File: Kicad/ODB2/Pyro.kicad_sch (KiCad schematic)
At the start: 35 parts

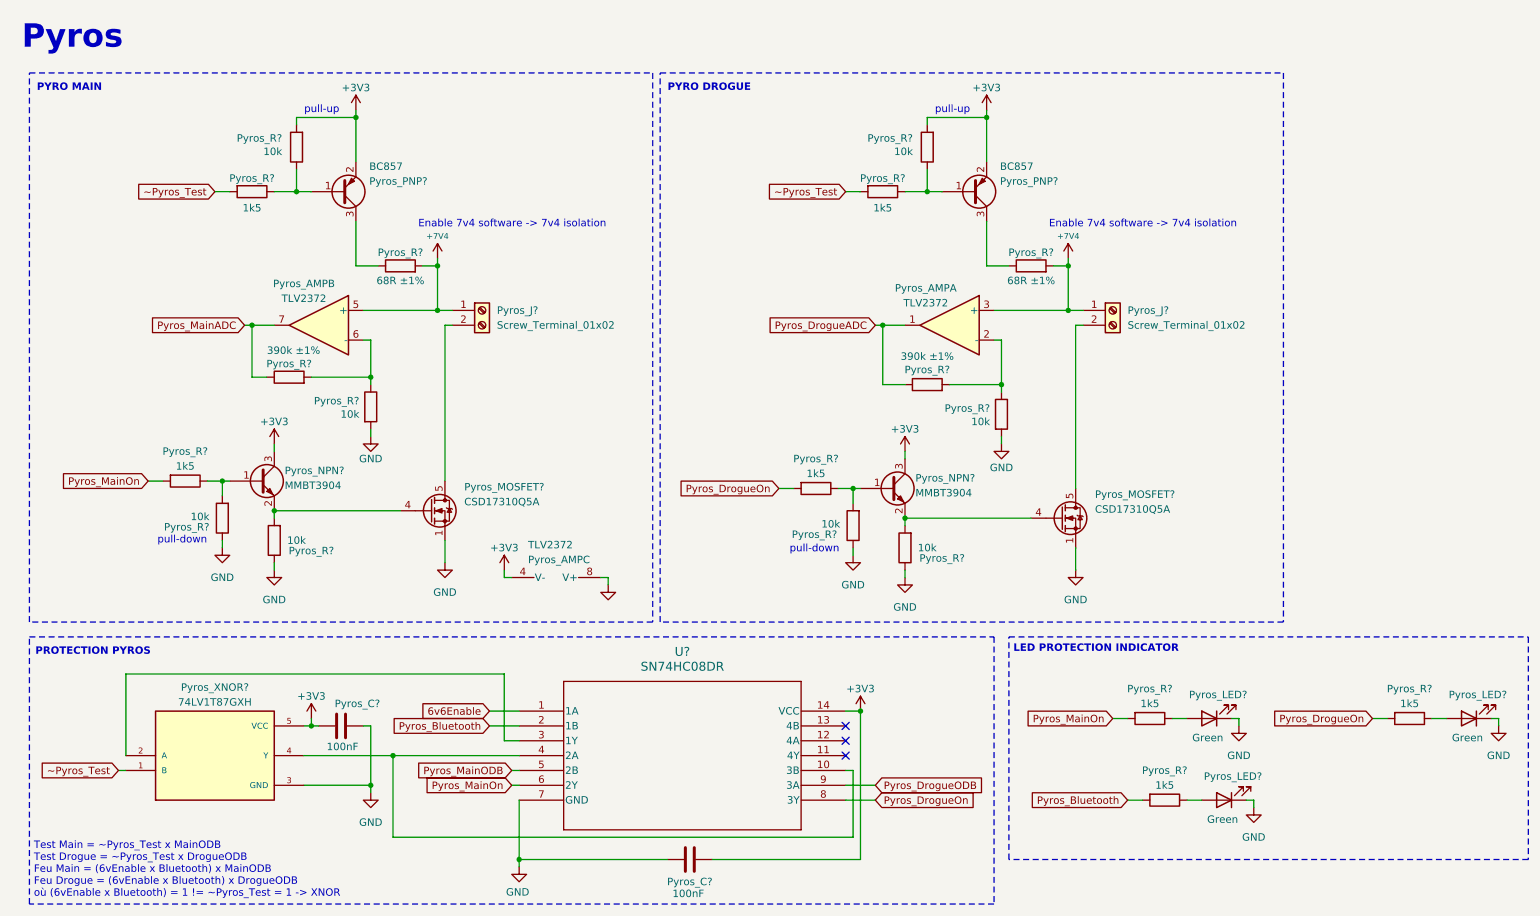
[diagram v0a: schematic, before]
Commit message: fix amp
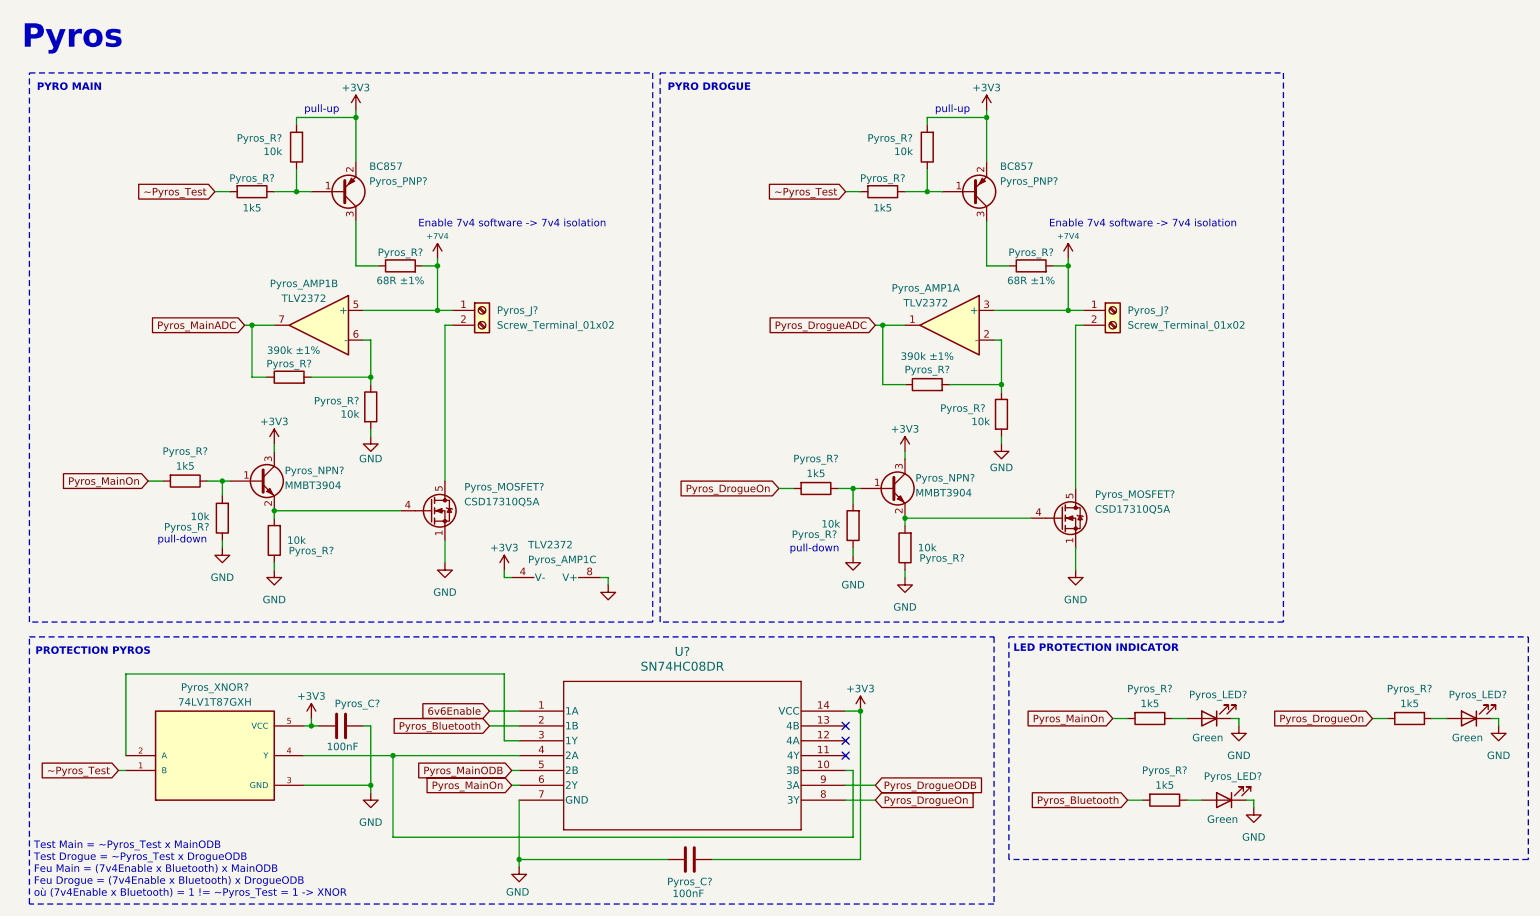
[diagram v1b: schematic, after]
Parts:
- Pyros_AMP1: renamed from Pyros_AMP; footprint (none) -> Package_SO:SOIC-8-1EP_3.9x4.9mm_P1.27mm_EP2.41x3.81mm
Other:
- note added: "Test Main = ~Pyros_Test x MainODB Test Drogue = ~Pyros_Test x DrogueODB Feu Main = (7v4Enable x Bluetooth) x MainODB Feu Drogue = (7v4Enable x Bluetooth) x DrogueODB où (7v4Enable x Bluetooth) = 1 != ~Pyros_Test = 1 -> XNOR"
- note removed: "Test Main = ~Pyros_Test x MainODB Test Drogue = ~Pyros_Test x DrogueODB Feu Main = (6vEnable x Bluetooth) x MainODB Feu Drogue = (6vEnable x Bluetooth) x DrogueODB où (6vEnable x Bluetooth) = 1 != ~Pyros_Test = 1 -> XNOR"
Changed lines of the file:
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@@
 		)
 	)
-	(text "Test Main = ~Pyros_Test x MainODB\nTest Drogue = ~Pyros_Test x DrogueODB\nFeu Main = (6vEnable x Bluetooth) x MainODB\nFeu Drogue = (6vEnable x Bluetooth) x DrogueODB\noù (6vEnable x Bluetooth) = 1 != ~Pyros_Test = 1 -> XNOR"
+	(text "Test Main = ~Pyros_Test x MainODB\nTest Drogue = ~Pyros_Test x DrogueODB\nFeu Main = (7v4Enable x Bluetooth) x MainODB\nFeu Drogue = (7v4Enable x Bluetooth) x DrogueODB\noù (7v4Enable x Bluetooth) = 1 != ~Pyros_Test = 1 -> XNOR"
 		(exclude_from_sim no)
 		(at 16.002 159.258 0)
@@
 		(on_board yes)
 		(dnp no)
-		(property "Reference" "Pyros_AMP"
+		(property "Reference" "Pyros_AMP1"
 			(at 100.584 106.172 90)
 			(effects
@@
 			)
 		)
-		(property "Footprint" ""
+		(property "Footprint" "Package_SO:SOIC-8-1EP_3.9x4.9mm_P1.27mm_EP2.41x3.81mm"
 			(at 105.41 106.68 0)
 			(effects
@@
 			(project ""
 				(path "/4b06c5d1-aa8b-48ed-8972-b43a60cfab78/8ab7427e-7183-4caa-ac8a-08b0bd412372"
-					(reference "Pyros_AMP")
+					(reference "Pyros_AMP1")
 					(unit 3)
 				)
@@
 		(dnp no)
 		(property "Reference" "Pyros_R?"
-			(at 175.768 80.264 0)
+			(at 175.006 80.264 0)
 			(effects
 				(font
@@
 		(on_board yes)
 		(dnp no)
-		(property "Reference" "#PWR077"
+		(property "Reference" "#PWR0105"
 			(at 85.09 58.42 0)
 			(effects
@@
 			(project "ODB2"
 				(path "/4b06c5d1-aa8b-48ed-8972-b43a60cfab78/8ab7427e-7183-4caa-ac8a-08b0bd412372"
-					(reference "#PWR077")
+					(reference "#PWR0105")
 					(unit 1)
 				)
@@
 		(on_board yes)
 		(dnp no)
-		(property "Reference" "Pyros_AMP"
+		(property "Reference" "Pyros_AMP1"
 			(at 168.656 59.69 0)
 			(effects
@@
 			)
 		)
-		(property "Footprint" ""
+		(property "Footprint" "Package_SO:SOIC-8-1EP_3.9x4.9mm_P1.27mm_EP2.41x3.81mm"
 			(at 172.72 66.04 0)
 			(effects
@@
 			(project ""
 				(path "/4b06c5d1-aa8b-48ed-8972-b43a60cfab78/8ab7427e-7183-4caa-ac8a-08b0bd412372"
-					(reference "Pyros_AMP")
+					(reference "Pyros_AMP1")
 					(unit 1)
 				)
@@
 		(on_board yes)
 		(dnp no)
-		(property "Reference" "Pyros_AMP"
+		(property "Reference" "Pyros_AMP1"
 			(at 62.23 58.928 0)
 			(effects
@@
 			)
 		)
-		(property "Footprint" ""
+		(property "Footprint" "Package_SO:SOIC-8-1EP_3.9x4.9mm_P1.27mm_EP2.41x3.81mm"
 			(at 64.77 66.04 0)
 			(effects
@@
 			(project ""
 				(path "/4b06c5d1-aa8b-48ed-8972-b43a60cfab78/8ab7427e-7183-4caa-ac8a-08b0bd412372"
-					(reference "Pyros_AMP")
+					(reference "Pyros_AMP1")
 					(unit 2)
 				)
